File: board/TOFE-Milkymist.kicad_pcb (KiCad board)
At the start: 2 copper layers, 110 x 111.3 mm, 116 parts, among them CON1 AUDIO_JACK_3535NG, CON2 AUDIO_JACK_3535NG, CON3 AUDIO_JACK_3535NG, CON4 AUDIO_JACK_3535NG, IC1 PC817, J1 DB9, K1 CONN_2, K2 CONN_2, K3 CONN_3, K4 CONN_3, K5 CONN_2, K6 CONN_2, K7 CONN_2, K8 CONN_2, P2 CONN_4X2, P4 CONN_6X2, P5 CONN_6X2, Q1 TRANSISTOR-NPN, SW1 SW_PUSH, SW2 SW_PUSH, SW3 SW_PUSH, SW4 SW_PUSH, U1 LM4550, U2 7805_N, U3 ST3232CDR, U4 SN74LVC1G17, U5 ISL83490, U6 IR-RX, U7 24AA01/24LC01B, U8 TIMVIDEOS-PCIE-8X, X1 CRYSTAL

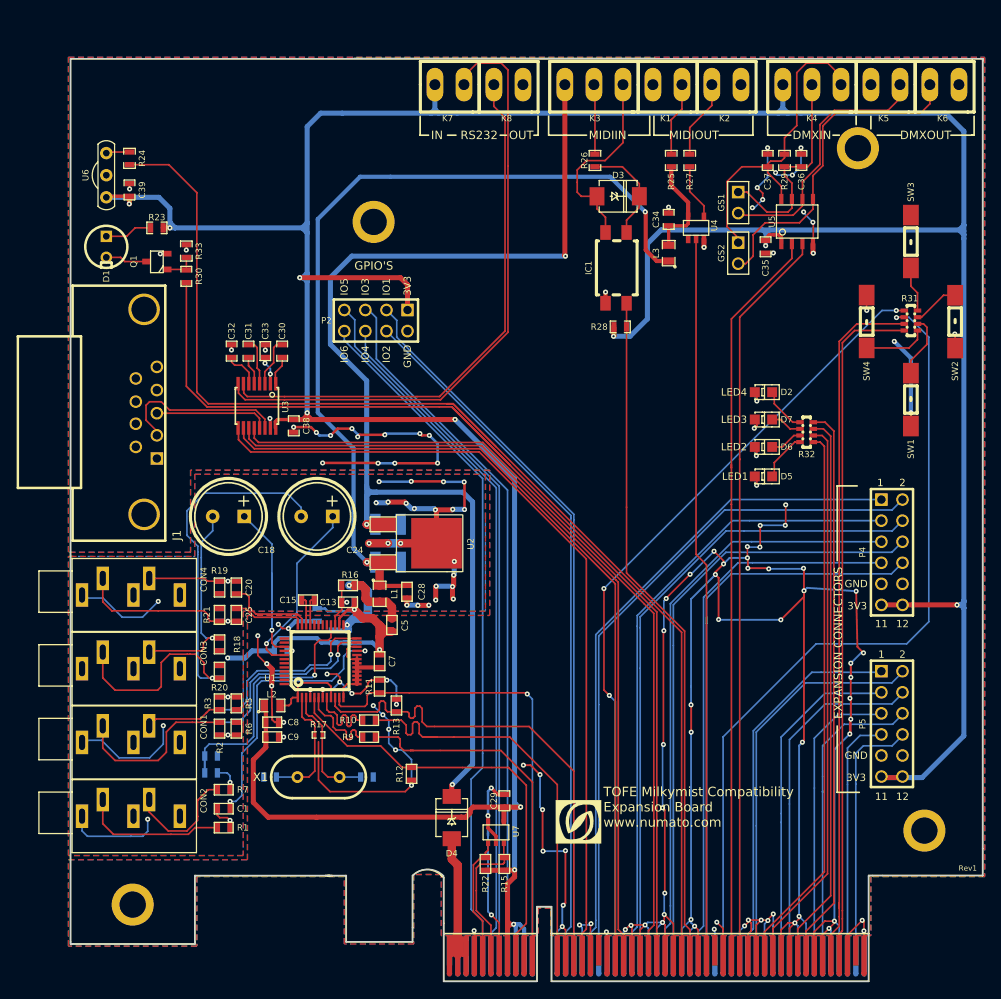
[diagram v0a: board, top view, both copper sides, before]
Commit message: More changes to mechanical holes.
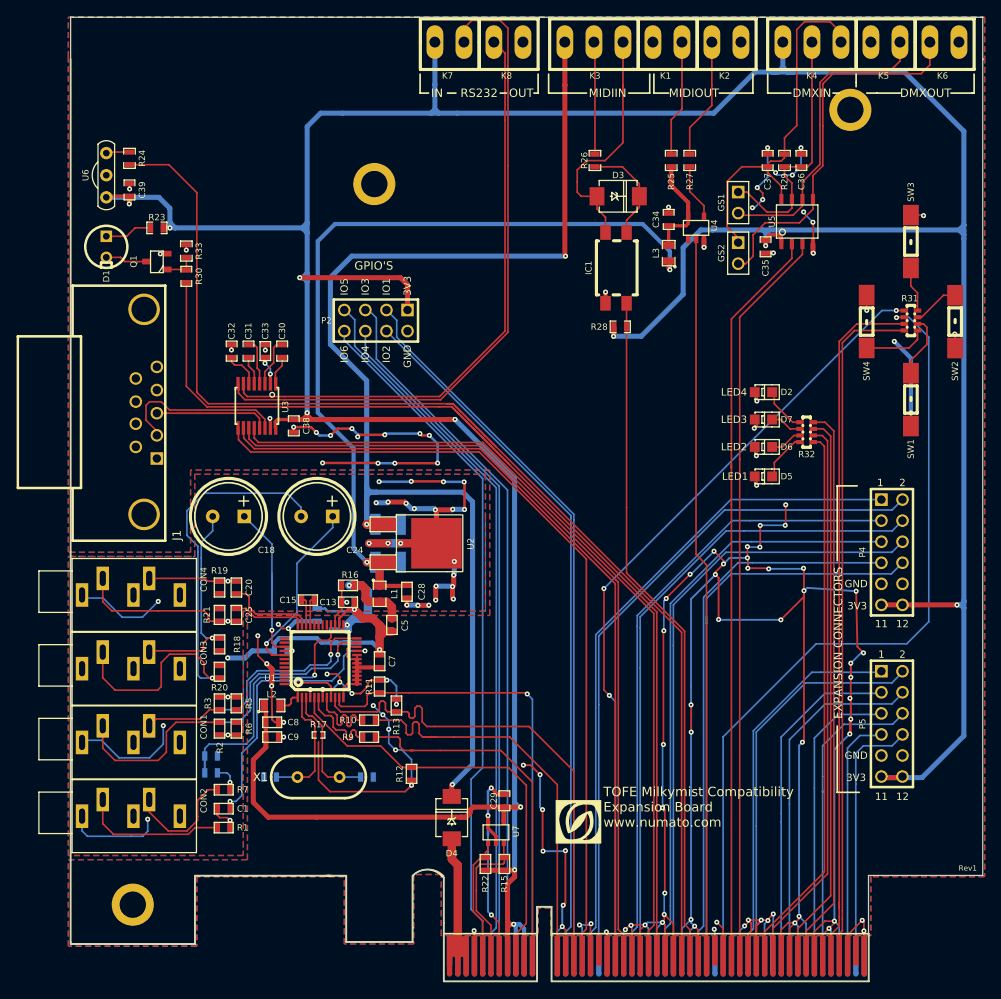
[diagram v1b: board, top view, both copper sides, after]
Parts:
- U8: footprint NumatoOpsis_PCIe_8X_HL_NW_110x110 -> NumatoOpsis_PCIe_8X_HL_NW_1
- moved U8 57.3 mm to (145.3, 148.3)
- moved K1 5.13 mm to (158.4, 35.0)
- moved K2 5.13 mm to (165.5, 35.0)
- moved K3 5.13 mm to (151.3, 35.0)
- moved K4 5.13 mm to (177.5, 35.0)
- moved K5 5.13 mm to (184.7, 35.0)
- moved K6 5.13 mm to (191.8, 35.0)
- moved K7 5.13 mm to (132.1, 35.0)
- moved K8 5.13 mm to (139.2, 35.0)
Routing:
- net /GND: track 596.1 -> 690.0 mm, vias 124 -> 125
- net /VCC3V3: track 492.0 -> 510.0 mm
- net /12V: track 36.4 -> 47.9 mm
- net /MIDI_IN_PIN5: track 23.9 -> 30.0 mm
- net /VCC5V0: track 104.4 -> 98.4 mm
- net /RS232-IN2: track 76.3 -> 81.8 mm
- net /DMX-DATA_OUT-: track 31.6 -> 37.1 mm
- net /DMX-DATA_OUT+: track 40.1 -> 45.5 mm
- net /DMX-DATA_IN-: track 25.9 -> 31.2 mm
- net /VCC12V: track 141.5 -> 146.7 mm
- net /MIDI_OUT_PIN4: track 8.92 -> 14.1 mm
- net /MIDI_OUT_PIN5: track 9.49 -> 14.6 mm
- net /MIDI_IN_PIN4: track 8.43 -> 13.6 mm
- net /RS232-OUT2: track 66.4 -> 71.5 mm
- net /DMX-DATA_IN+: track 39.2 -> 44.3 mm
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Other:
- board size 110 x 111.3 mm -> 110 x 116.3 mm
